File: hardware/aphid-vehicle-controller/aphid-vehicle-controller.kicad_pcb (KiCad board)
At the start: 4 copper layers, 85 x 107.5 mm, 139 parts, among them J1 MONITOR UART, J2 ModICE ME-MX 24, J3 MAIN_SWD, J4 MONITOR_SWD, U1 STM32G491CETx, U2 LD1117S33TR_SOT223, U3 LMR33630BDDA, U4 TJA1042T-3, U5 TJA1042T-3, U6 TJA1042T-3, U7 STM32G431KBTx, U8 BTS6143D, Y1 8 MHz, Y2 8 MHz

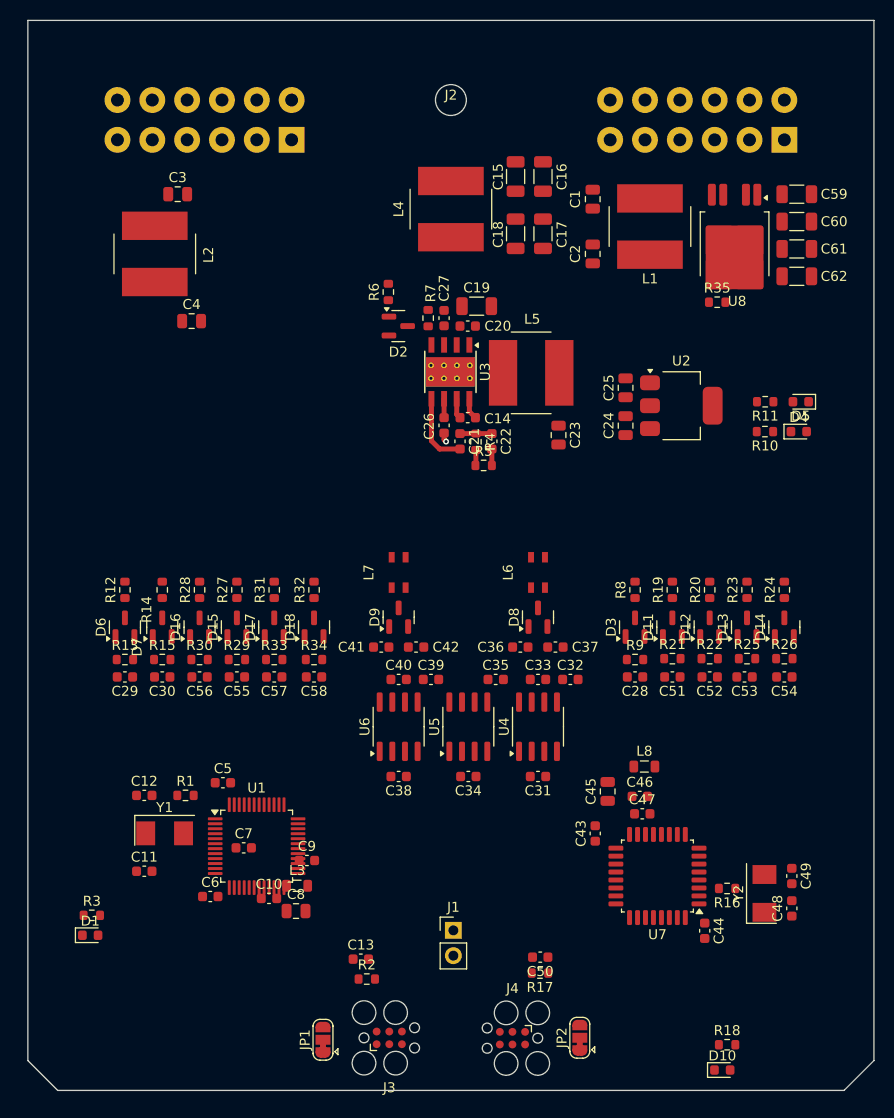
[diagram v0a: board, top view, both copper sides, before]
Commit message: worked on vcu pcb
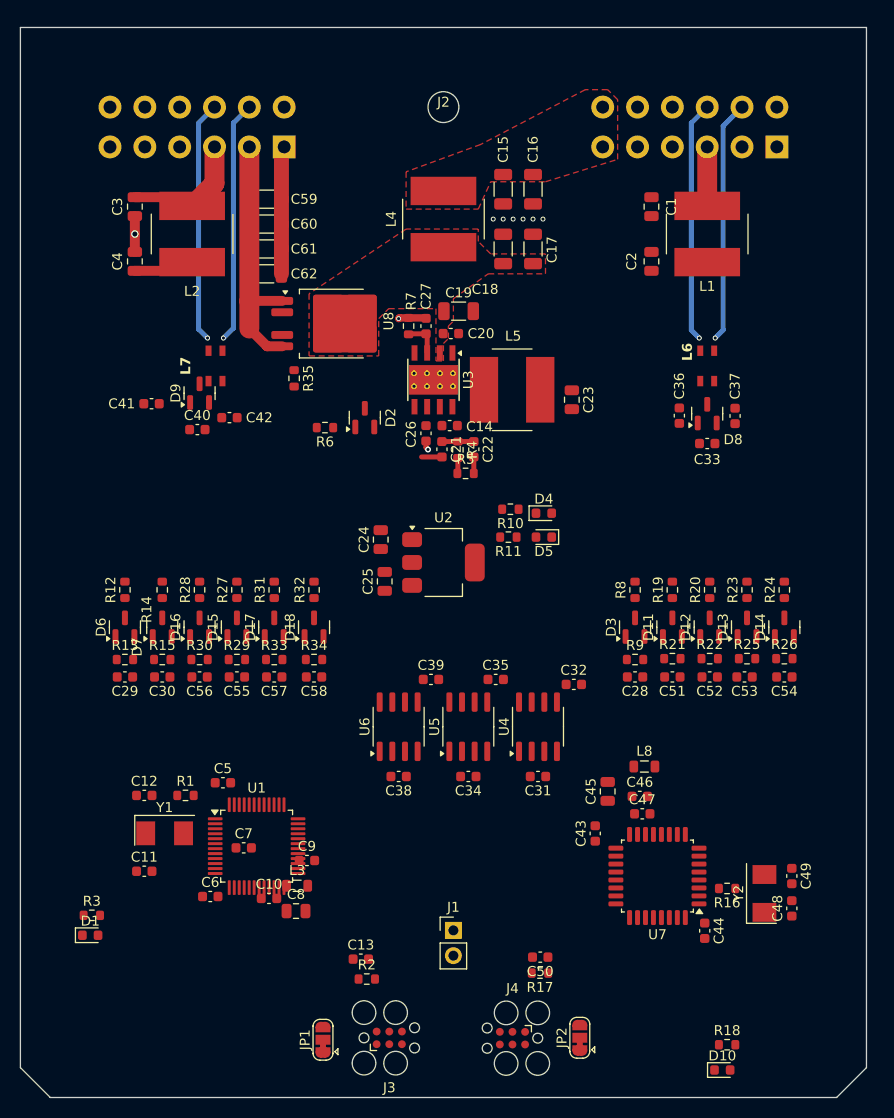
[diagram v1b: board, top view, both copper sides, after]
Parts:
- moved C59 53.3 mm to (120.8, 59.2)
- moved C60 53.3 mm to (120.8, 61.8)
- moved C62 53.3 mm to (120.8, 66.8)
- moved C61 53.2 mm to (120.8, 64.2)
- moved R35 43.2 mm to (123.5, 77.2), turned to -90 degrees
- moved U8 41.2 mm to (127.3, 71.8), turned to 0 degrees
- moved C41 33.6 mm to (109.2, 79.8)
- moved C40 32.2 mm to (113.8, 82.4)
- moved C25 31.0 mm to (132.6, 97.7)
- moved D9 30.1 mm to (114.0, 78.7)
- moved C42 29.7 mm to (117.0, 81.2)
- moved C37 29.4 mm to (167.8, 81.0), turned to 90 degrees
- moved D5 29.2 mm to (148.6, 93.2)
- moved C33 29.2 mm to (165.0, 83.8)
- moved R11 29.2 mm to (145.0, 93.2)
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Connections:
- J2 pad 14: GND -> /Connectors/HIGH_SIDE_DRIVE
- J2 pad 2: /Connectors/HIGH_SIDE_DRIVE -> GND
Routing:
- net /Connectors/HIGH_SIDE_DRIVE: track 0.00 -> 25.6 mm
- net /CAN/CAN1_LOW: track 0.00 -> 24.3 mm, vias 0 -> 1
- net /CAN/CAN2_LOW: track 0.00 -> 24.3 mm, vias 0 -> 1
- net /CAN/CAN2_HIGH: track 0.00 -> 24.2 mm, vias 0 -> 1
- net /CAN/CAN1_HIGH: track 0.00 -> 24.2 mm, vias 0 -> 1
- net GND: track 2.58 -> 21.8 mm, vias 1 -> 3
- net Net-(J2B-R3): track 0.00 -> 13.0 mm
- net +5V: track 3.20 -> 9.31 mm
- net Net-(J2A-L3): track 0.00 -> 5.92 mm
- net Net-(U3-FB): track 9.01 -> 3.62 mm
- net Net-(U3-EN): track 0.00 -> 3.74 mm
- net Net-(U3-SW): track 2.15 -> 0.00 mm
- net Net-(U3-BOOT): track 2.04 -> 0.00 mm
- net Net-(U3-VCC): track 1.90 -> 0.00 mm
- net (no net): vias 0 -> 6
- added copper zone on F.Cu, net +12V
- added copper zone on F.Cu, net /Connectors/VIN
